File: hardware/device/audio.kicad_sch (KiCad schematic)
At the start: 33 parts, among them J10 MIDI_OUT, J6 LINE_IN, J7 LINE_OUT, J9 MIDI_IN, U24 WM8904CGEFL/RV, U28 TPS560200

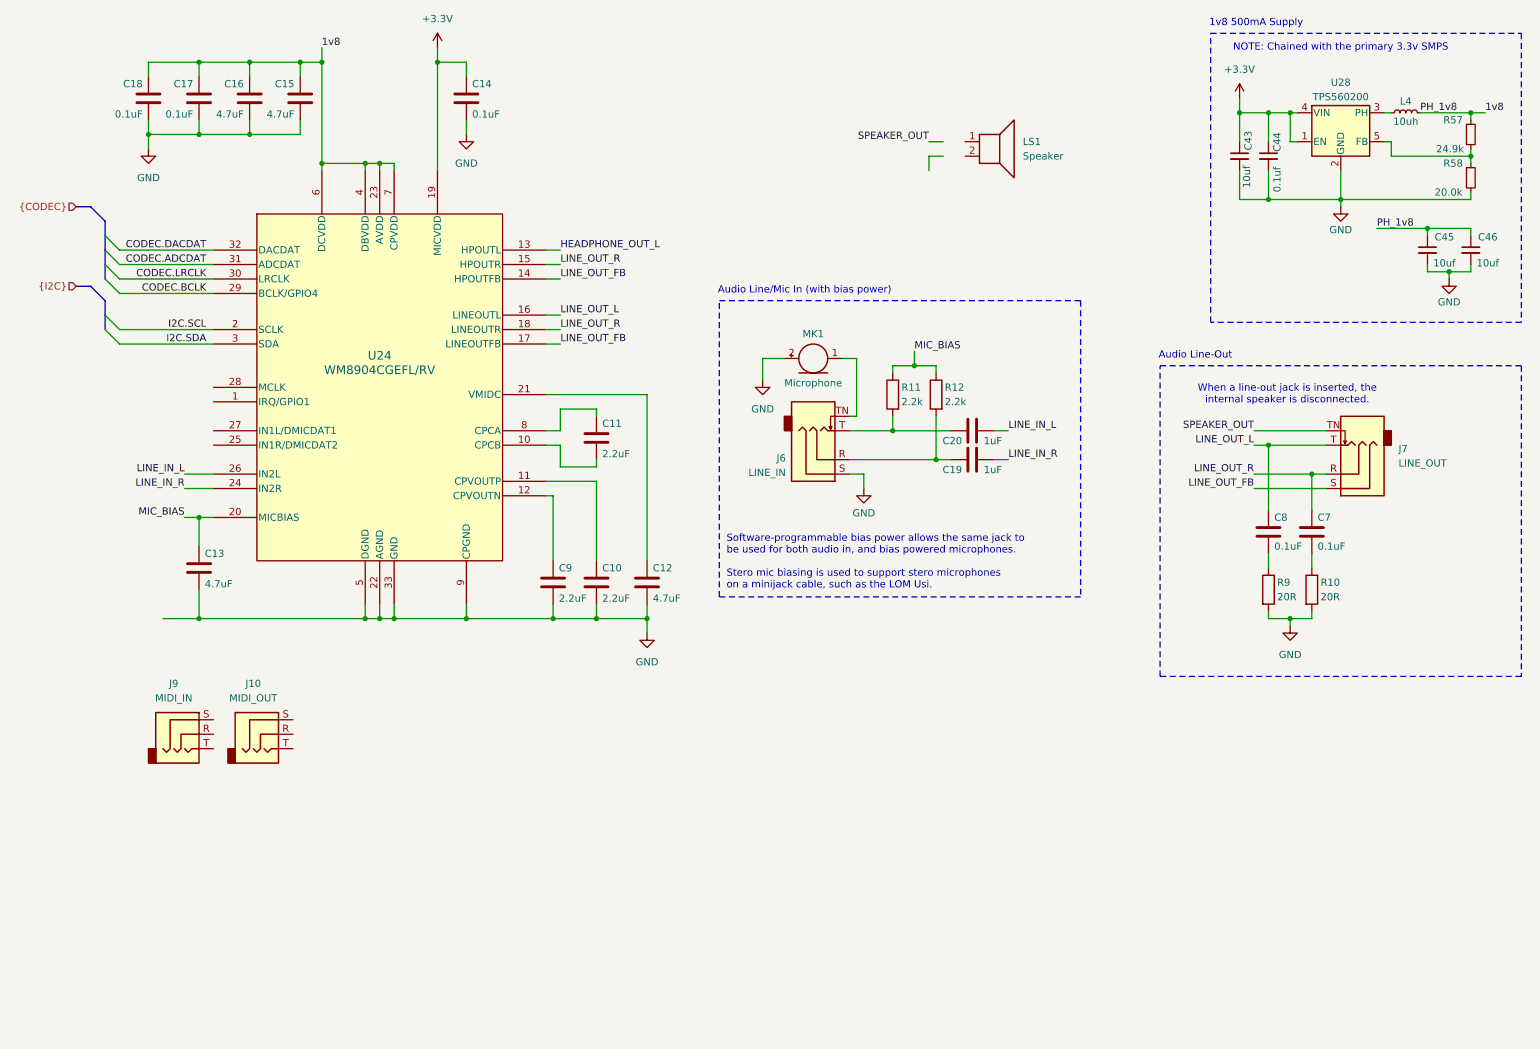
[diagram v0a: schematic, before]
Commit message: feat: various layouts, changed SDRAM to BGA
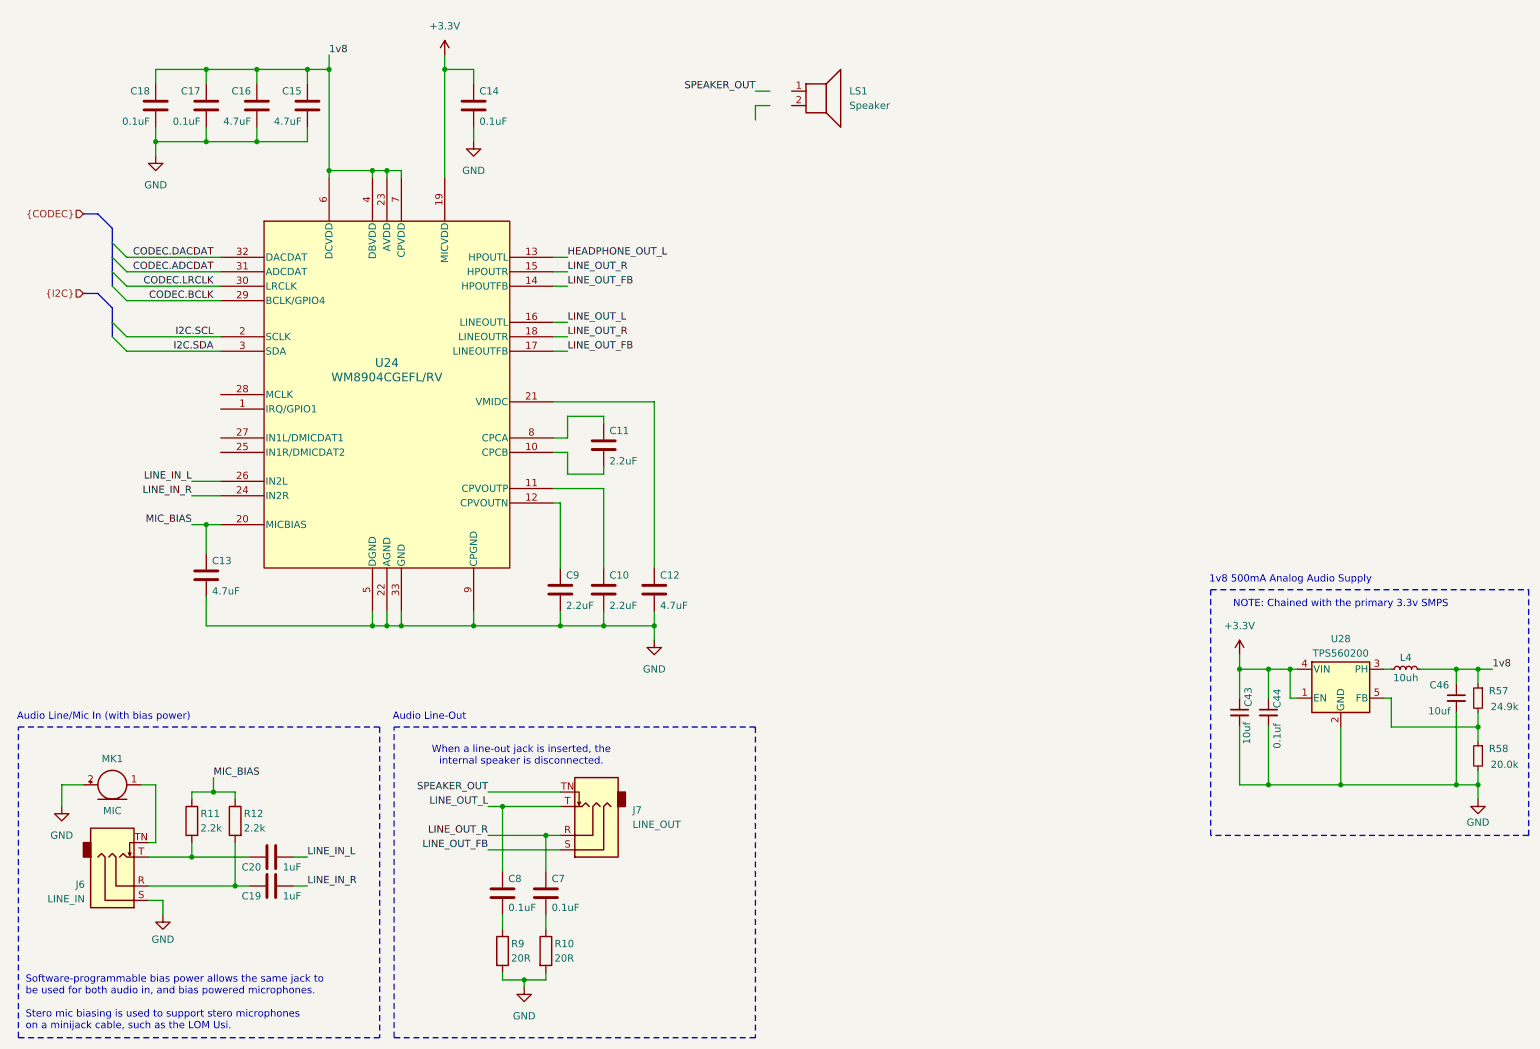
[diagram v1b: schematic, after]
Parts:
- removed C45: 10uf, Capacitor_SMD:C_0402_1005Metric_Pad0.74x0.62mm_HandSolder, symbol Device:C_Small
- removed J10: MIDI_OUT, Connector_Audio:Jack_3.5mm_CUI_SJ-3523-SMT_Horizontal, symbol Connector_Audio:AudioJack3
- removed J9: MIDI_IN, Connector_Audio:Jack_3.5mm_CUI_SJ-3523-SMT_Horizontal, symbol Connector_Audio:AudioJack3
- MK1: value Microphone -> MIC
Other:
- note added: "1v8 500mA Analog Audio Supply"
- note removed: "1v8 500mA Supply"
- moved on the sheet: C10, C11, C12, C13, C14, C15, C16, C17, C18, C19, C20, C43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
